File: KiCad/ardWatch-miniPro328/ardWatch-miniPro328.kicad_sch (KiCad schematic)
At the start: 8 parts, among them J1 2-pin_power_input_header, U1 Arduino_Mini_Pro, U2 KY-040_Rotary_Encoder, U3 ST7735_1.8"_TFT_128x160, U4 DS3231_RTC_module

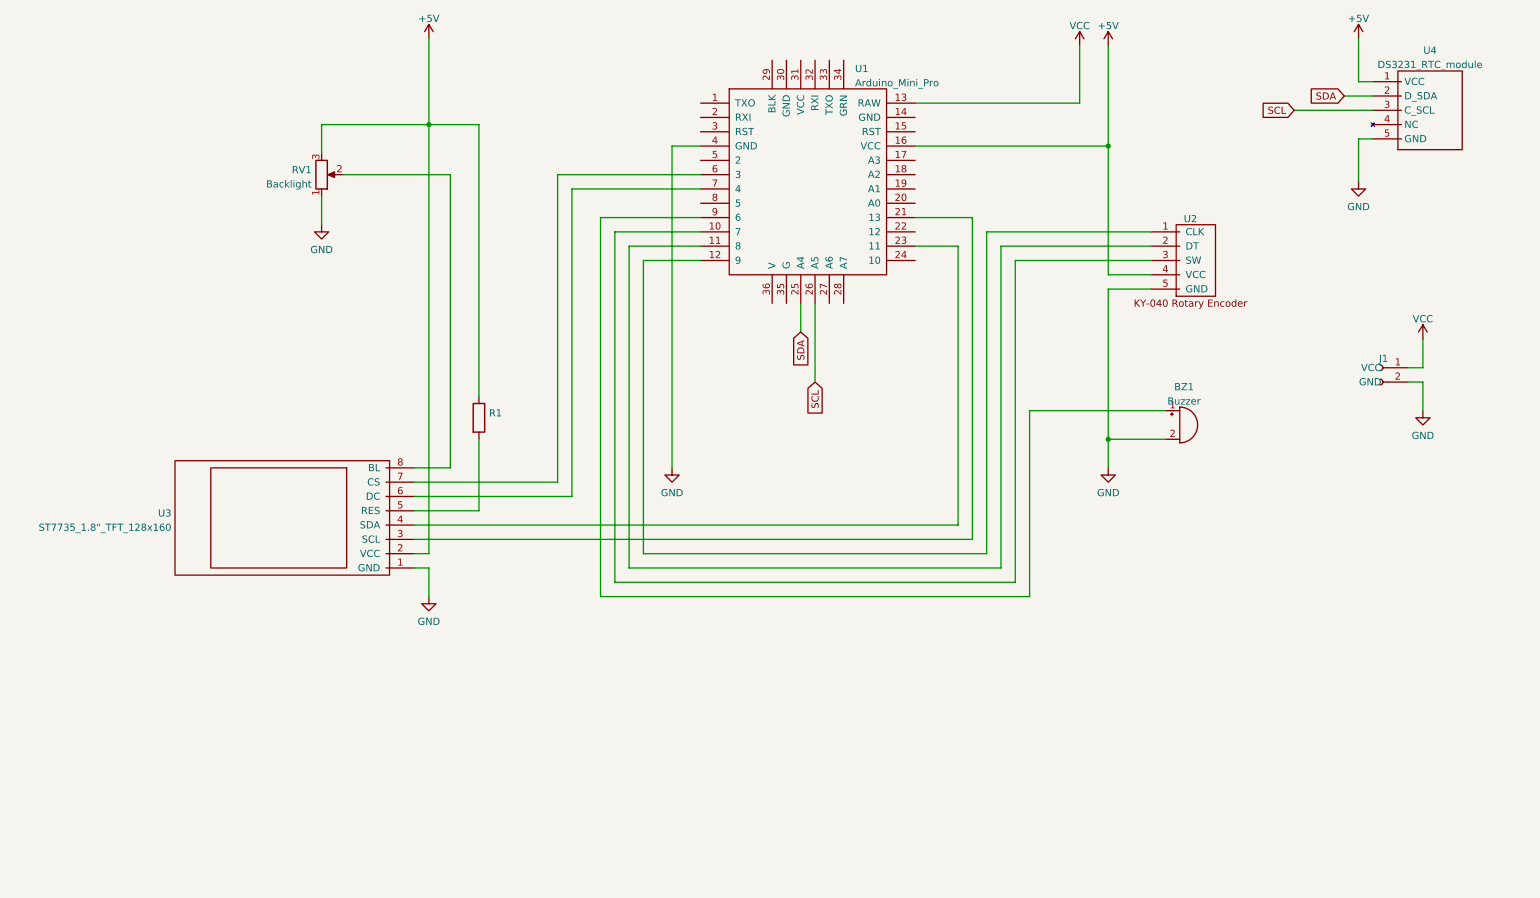
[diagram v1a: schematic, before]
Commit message: new layout
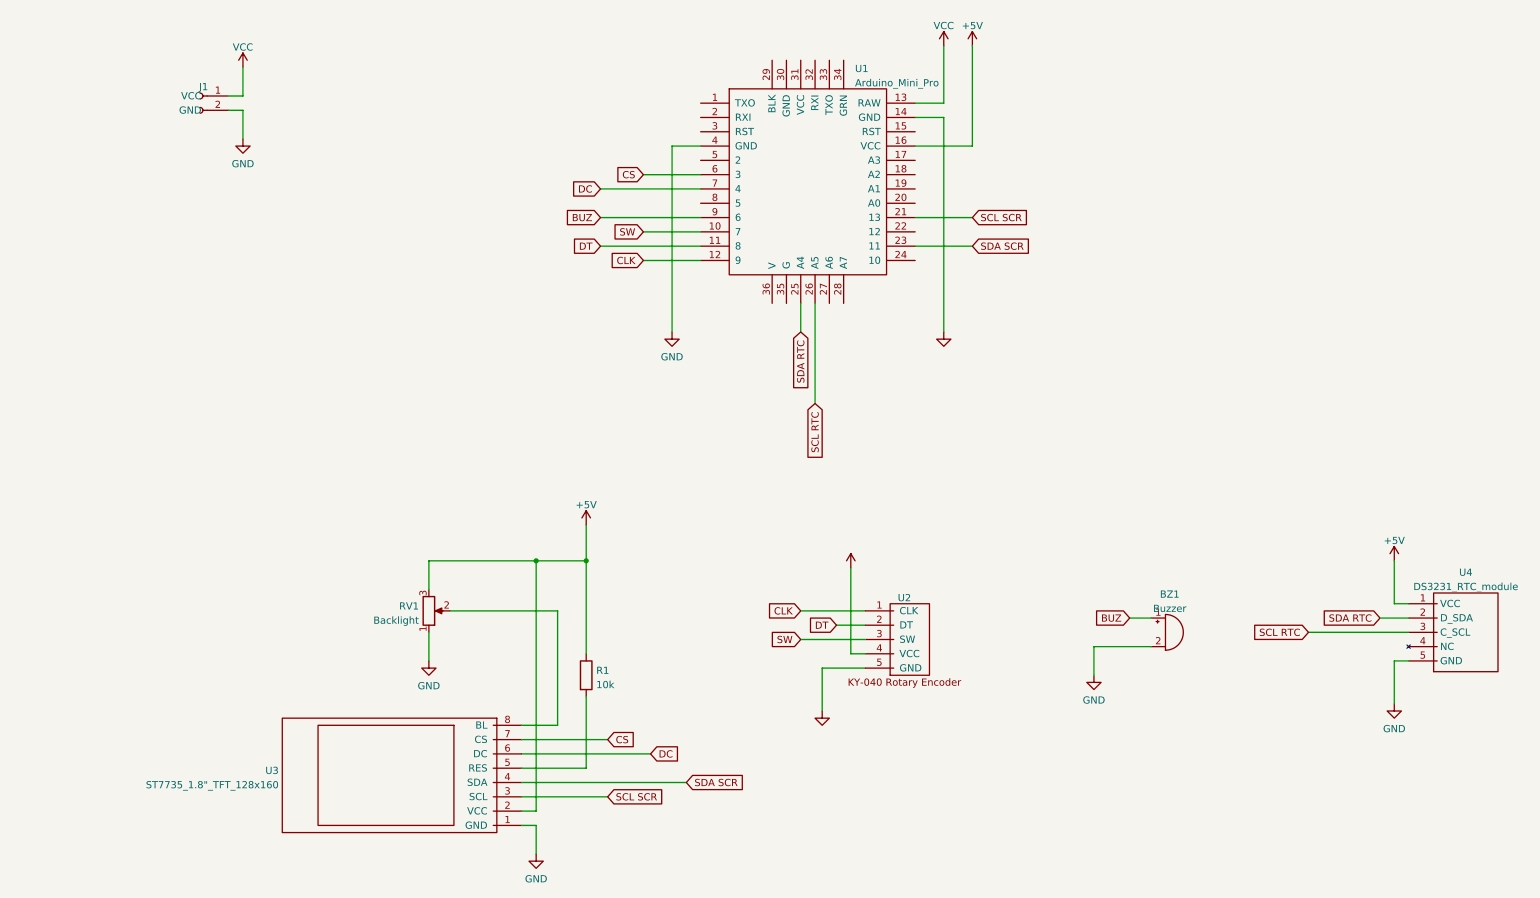
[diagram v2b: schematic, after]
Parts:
- R1: value (none) -> 10k; footprint (none) -> My_Misc:R_Axial_DIN0207_L6.3mm_D2.5mm_P10.16mm_Horizontal_larger_pads
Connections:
- net GND: now also U1.14 (GND)
- net SW: now reaches U1.10 (7), U2.3 (SW)
- net DT: now reaches U1.11 (8), U2.2 (DT)
- net CLK: now reaches U1.12 (9), U2.1 (CLK)
- net SCL SCR: now reaches U1.21 (13), U3.3 (SCL)
- net SDA SCR: now reaches U1.23 (11), U3.4 (SDA)
- net CS: now reaches U1.6 (3), U3.7 (CS)
- net DC: now reaches U1.7 (4), U3.6 (DC)
- net BUZ: now reaches BZ1.1 (-), U1.9 (6)
- net SCL renamed SCL RTC
- net SDA renamed SDA RTC
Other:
- moved on the sheet: BZ1, J1, R1, RV1, U2, U3, U4
